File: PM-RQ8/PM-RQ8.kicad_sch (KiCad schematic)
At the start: 33 parts, among them J1 2EDGK-5.08-02P, J10 2EDGR-5.08-18P, J11 Shunt 2.54 Open Top, J12 PinHeader_P2.54_01x03_SMD_Str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, J13 PinHeader_P2.54_01x03_SMD_Str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, J14 PinHeader_P2.54_01x03_SMD_Str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, J15 FemaleHeader P2.54 02x08 THT 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, J16 Shunt 2.54 Open Top, J17 Shunt 2.54 Open Top, J18 2EDGK-5.08-02P, J2 2EDGK-5.08-02P, J3 2EDGK-5.08-02P, J4 2EDGK-5.08-02P, J5 2EDGK-5.08-02P, J6 2EDGK-5.08-02P, J7 2EDGK-5.08-02P, J8 2EDGK-5.08-02P, J9 Conn_01x04_Pin, K1 G5NB-1A-E-DC5, K2 G5NB-1A-E-DC5, K3 G5NB-1A-E-DC5, K4 G5NB-1A-E-DC5, K5 G5NB-1A-E-DC5, K6 G5NB-1A-E-DC5, K7 G5NB-1A-E-DC5, K8 G5NB-1A-E-DC5, U1 ULN2803A, U2 PCA9555PW, U4 64900001039

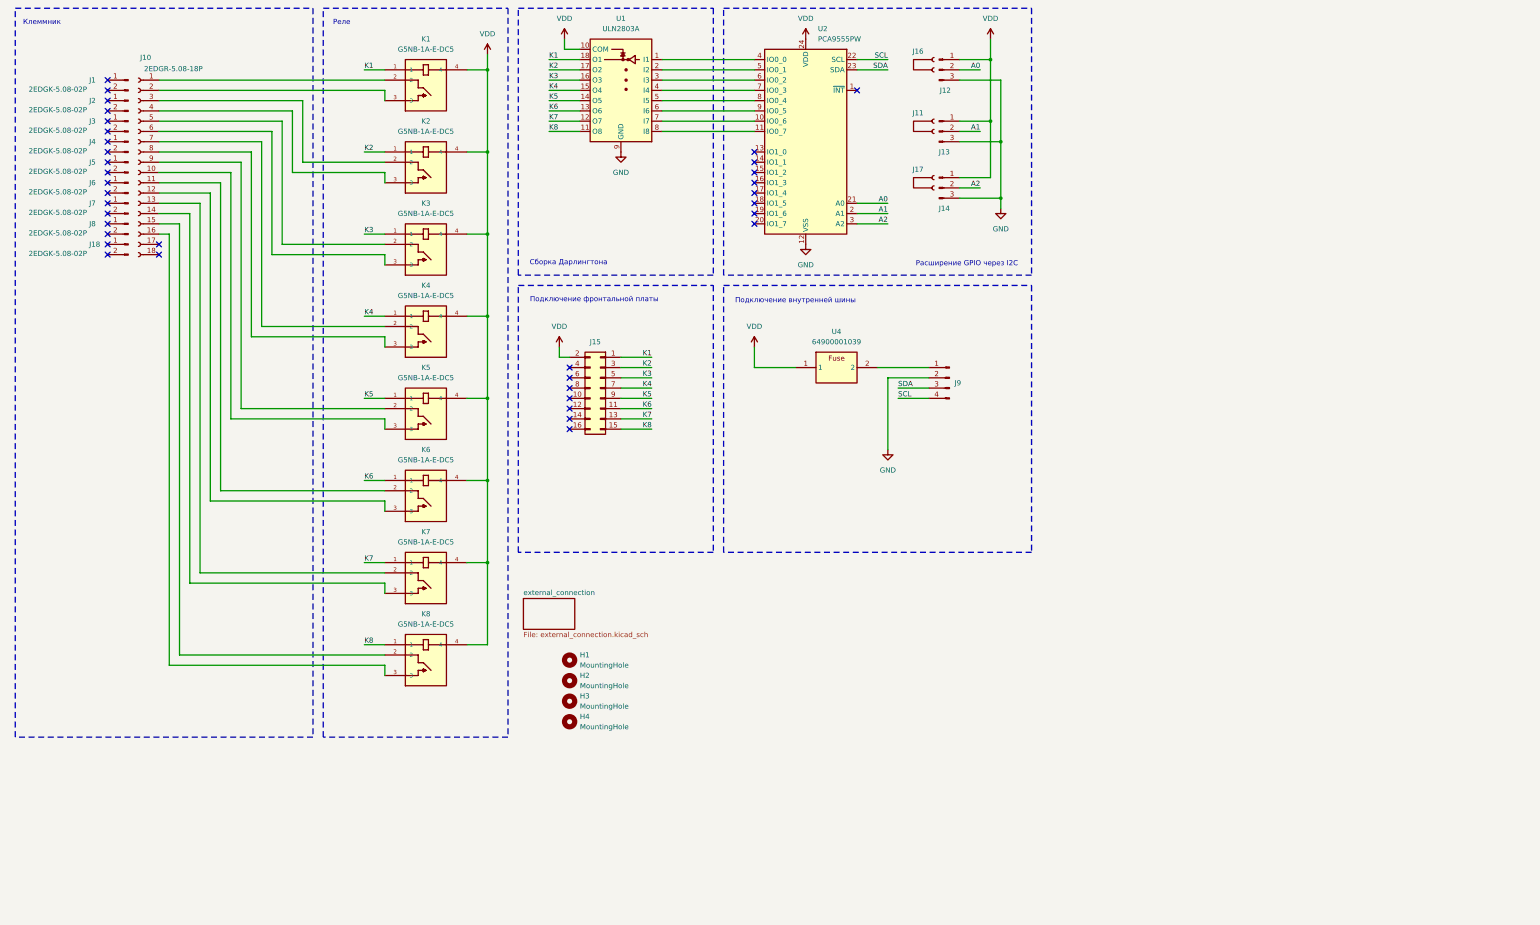
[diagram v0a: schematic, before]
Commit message: send to nextpcb
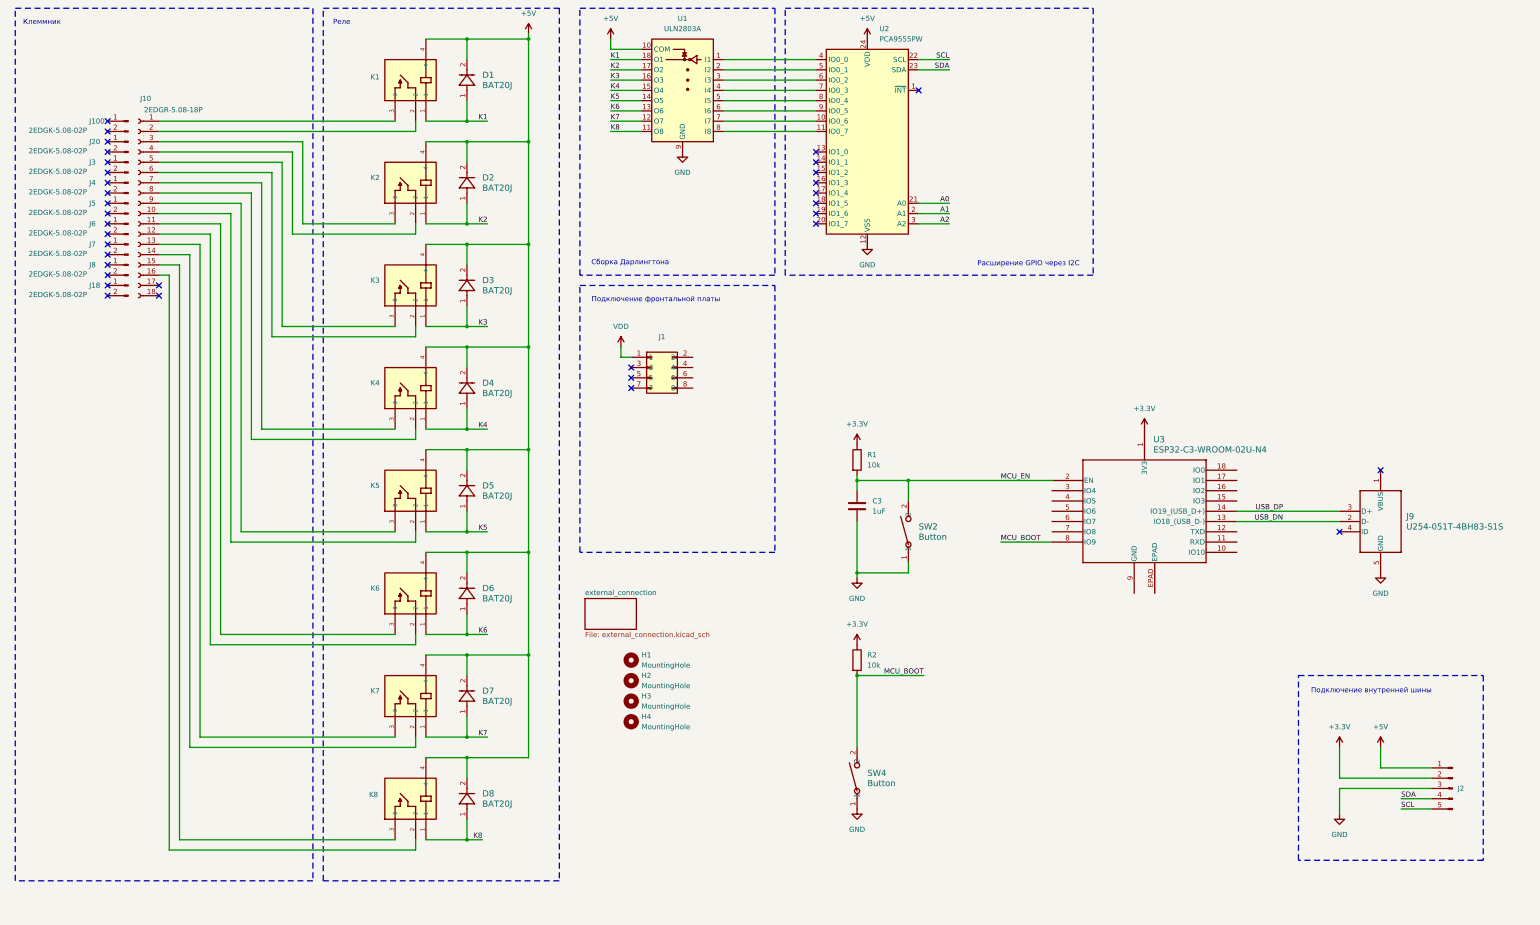
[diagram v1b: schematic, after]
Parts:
- removed J11, J16, J17: Shunt 2.54 Open Top, symbol kicad_inventree_lib:Shunt 2.54 Open Top
- removed J12, J13, J14: PinHeader_P2.54_01x03_SMD_Straight, Connector_PinHeader_2.54mm:PinHeader_1x03_P2.54mm_Vertical_SMD_Pin1Left, symbol kicad_inventree_lib:PinHeader P2.54 01x03 SMD Straight
- removed J15: FemaleHeader P2.54 02x08 THT Straight, Connector_PinSocket_2.54mm:PinSocket_2x08_P2.54mm_Vertical, symbol kicad_inventree_lib:FemaleHeader P2.54 02x08 THT Straight
- removed J9: Conn_01x04_Pin, Connector_PinHeader_2.54mm:PinHeader_1x04_P2.54mm_Horizontal, symbol kicad_inventree_lib:PinHeader P2.54 01x04 THT Angle
- removed U4: 64900001039, NextPCB:Fuseholder, symbol kicad_inventree_lib:Fuseholder
- added C3: 1uF, Capacitor_SMD:C_1206_3216Metric_Pad1.33x1.80mm_HandSolder, symbol kicad_inventree_lib:C_1uF_50V_1206
- added D1, D2, D3, D4, D5, D6, D7, D8: BAT20J, kicad_inventree_lib:SOD-323_STM-M, symbol kicad_inventree_lib:BAT20J
- added J1: ~, kicad_inventree_lib:PM-front-02x04, symbol kicad_inventree_lib:PM-front-02x04
- added J2: PinHeader_01x05_P2.54_THT_angle, Connector_PinHeader_2.54mm:PinHeader_1x05_P2.54mm_Horizontal, symbol kicad_inventree_lib:PinHeader_01x05_P2.54_THT_angle
- added J9: U254-051T-4BH83-S1S, kicad_inventree_lib:CONN5_H83-S1S_XKB, symbol kicad_inventree_lib:XKG_U254-051T-4BH83-S1S
- added R1, R2: 10k, Resistor_SMD:R_1206_3216Metric_Pad1.30x1.75mm_HandSolder, symbol kicad_inventree_lib:R_10k_1206_1%
- added SW2, SW4: Button, kicad_inventree_lib:SW_TS-1088_XNP-M, symbol kicad_inventree_lib:TS-1088-AR02016
- added U3: ESP32-C3-WROOM-02U-N4, ESP32-C3-WROOM-02U_EXP, symbol kicad_inventree_lib:ESP32-C3-WROOM-02U-N4
- renumbered J1 to J100, J2 to J20
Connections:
- net GND: now also C3.2, J2.3 (Pin_3), J9.5 (GND), SW2.1, SW4.1
- net K1: now also D1.1
- net K2: now also D2.1
- net K3: now also D3.1
- net K4: now also D4.1
- net K5: now also D5.1
- net K6: now also D6.1
- net K7: now also D7.1
- net K8: now also D8.1
- net SCL: now also J2.5 (Pin_5)
- net SDA: now also J2.4 (Pin_4)
- net VDD: now also J1.1; no longer K1.4, K2.4, K3.4, K4.4, K5.4, K6.4, K7.4, K8.4, U1.10 (COM), U2.24 (VDD)
- net at K5.2: now also J10.10 (Pin_10); no longer J10.9 (Pin_9)
- net at K5.3: now also J10.9 (Pin_9); no longer J10.10 (Pin_10)
- net at K3.2: now also J10.6 (Pin_6); no longer J10.5 (Pin_5)
- net at K3.3: now also J10.5 (Pin_5); no longer J10.6 (Pin_6)
- net at K8.2: now also J10.16 (Pin_16); no longer J10.15 (Pin_15)
- net at K8.3: now also J10.15 (Pin_15); no longer J10.16 (Pin_16)
- net at K2.2: now also J10.4 (Pin_4); no longer J10.3 (Pin_3)
- net at K2.3: now also J10.3 (Pin_3); no longer J10.4 (Pin_4)
- net at K4.2: now also J10.8 (Pin_8); no longer J10.7 (Pin_7)
- net at K4.3: now also J10.7 (Pin_7); no longer J10.8 (Pin_8)
- net at K1.2: now also J10.2 (Pin_2); no longer J10.1 (Pin_1)
- net at K1.3: now also J10.1 (Pin_1); no longer J10.2 (Pin_2)
- net at J10.11 (Pin_11): now also K6.3; no longer K6.2
- net at J10.12 (Pin_12): now also K6.2; no longer K6.3
- net at J10.13 (Pin_13): now also K7.3; no longer K7.2
- net at J10.14 (Pin_14): now also K7.2; no longer K7.3
- new net +3.3V: J2.2 (Pin_2), R1.1, R2.1, U3.1 (3V3)
- new net +5V: D1.2, D2.2, D3.2, D4.2, D5.2, D6.2, D7.2, D8.2, J2.1 (Pin_1), K1.4, K2.4, K3.4, K4.4, K5.4, K6.4, K7.4, K8.4, U1.10 (COM), U2.24 (VDD)
- new net MCU_BOOT: R2.2, SW4.2, U3.8 (IO9)
- new net MCU_EN: C3.1, R1.2, SW2.2, U3.2 (EN)
- new net USB_DN: J9.2 (D-), U3.13 (IO18_(USB_D-))
- new net USB_DP: J9.3 (D+), U3.14 (IO19_(USB_D+))
- no-connect marks 36 -> 34
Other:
- moved on the sheet: H1, H2, H3, H4, J10, J100, J18, J20, J3, J4, J5, J6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

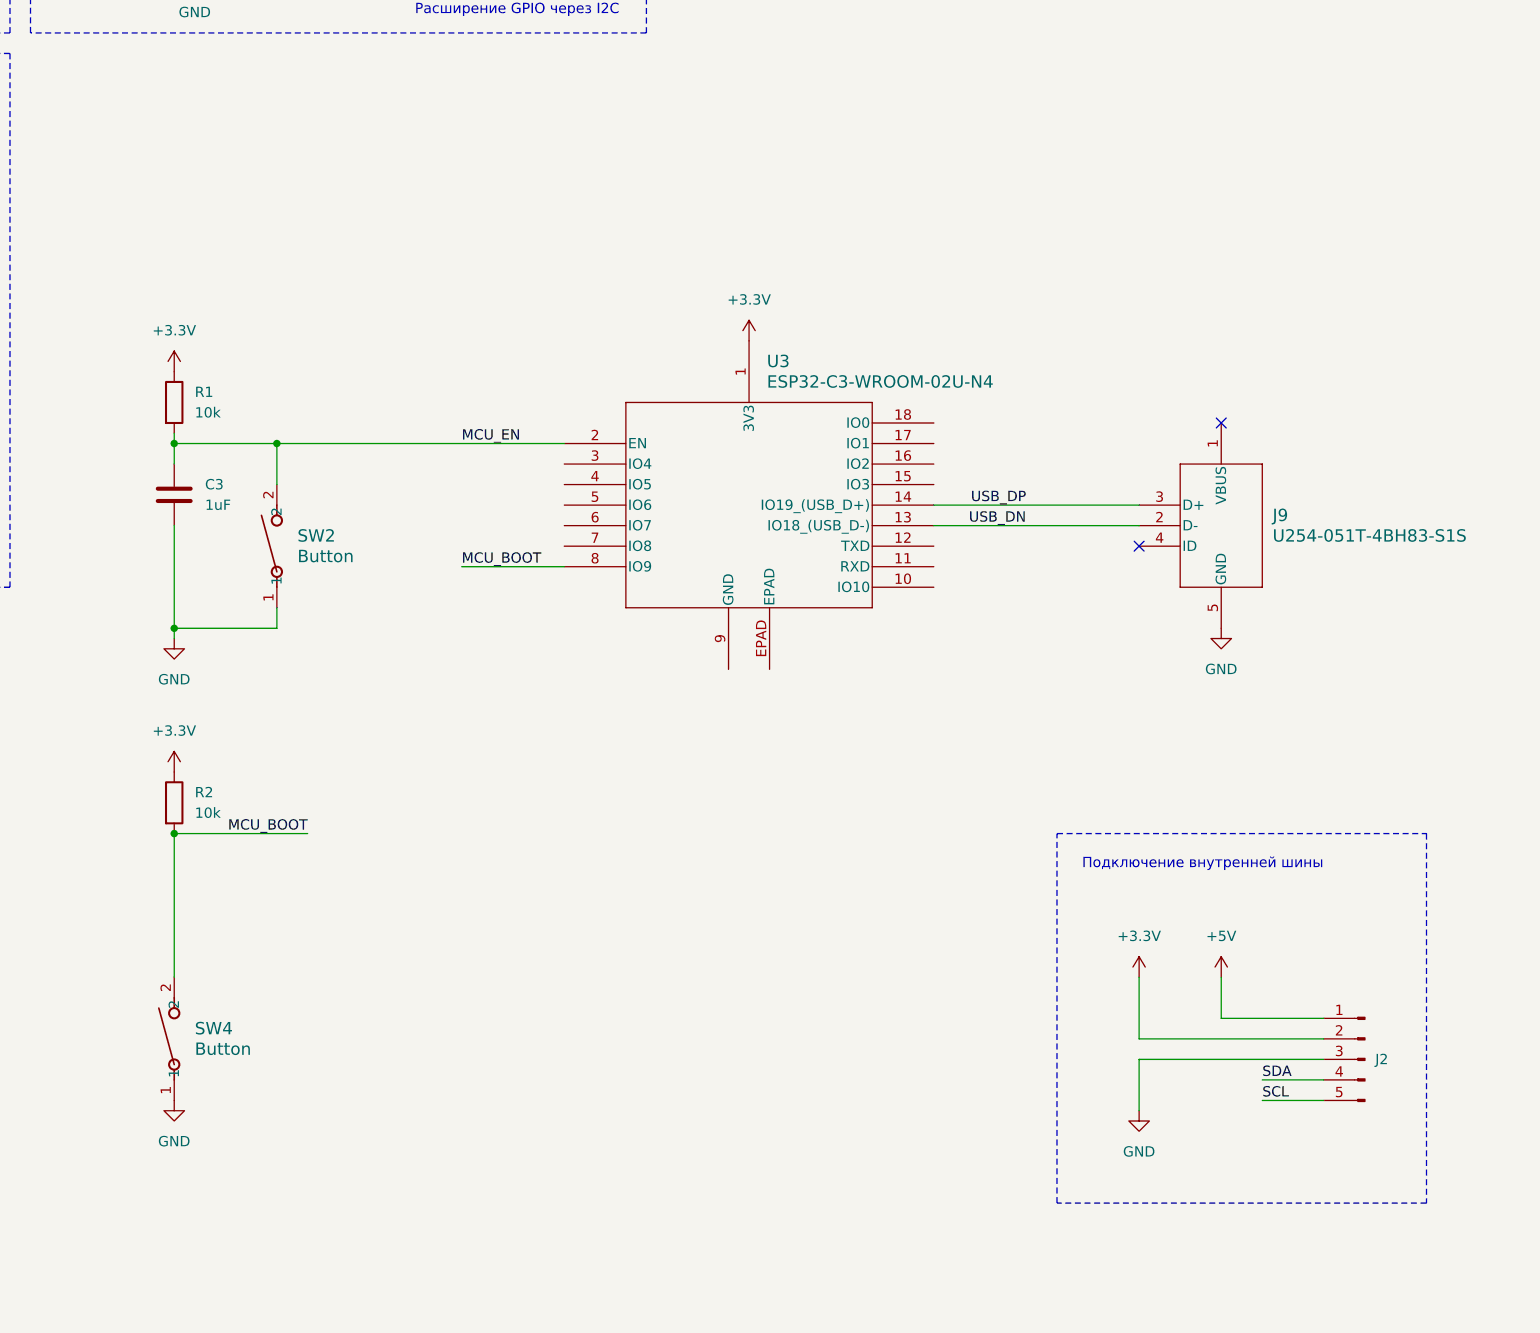
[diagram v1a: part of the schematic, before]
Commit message: PM-PS
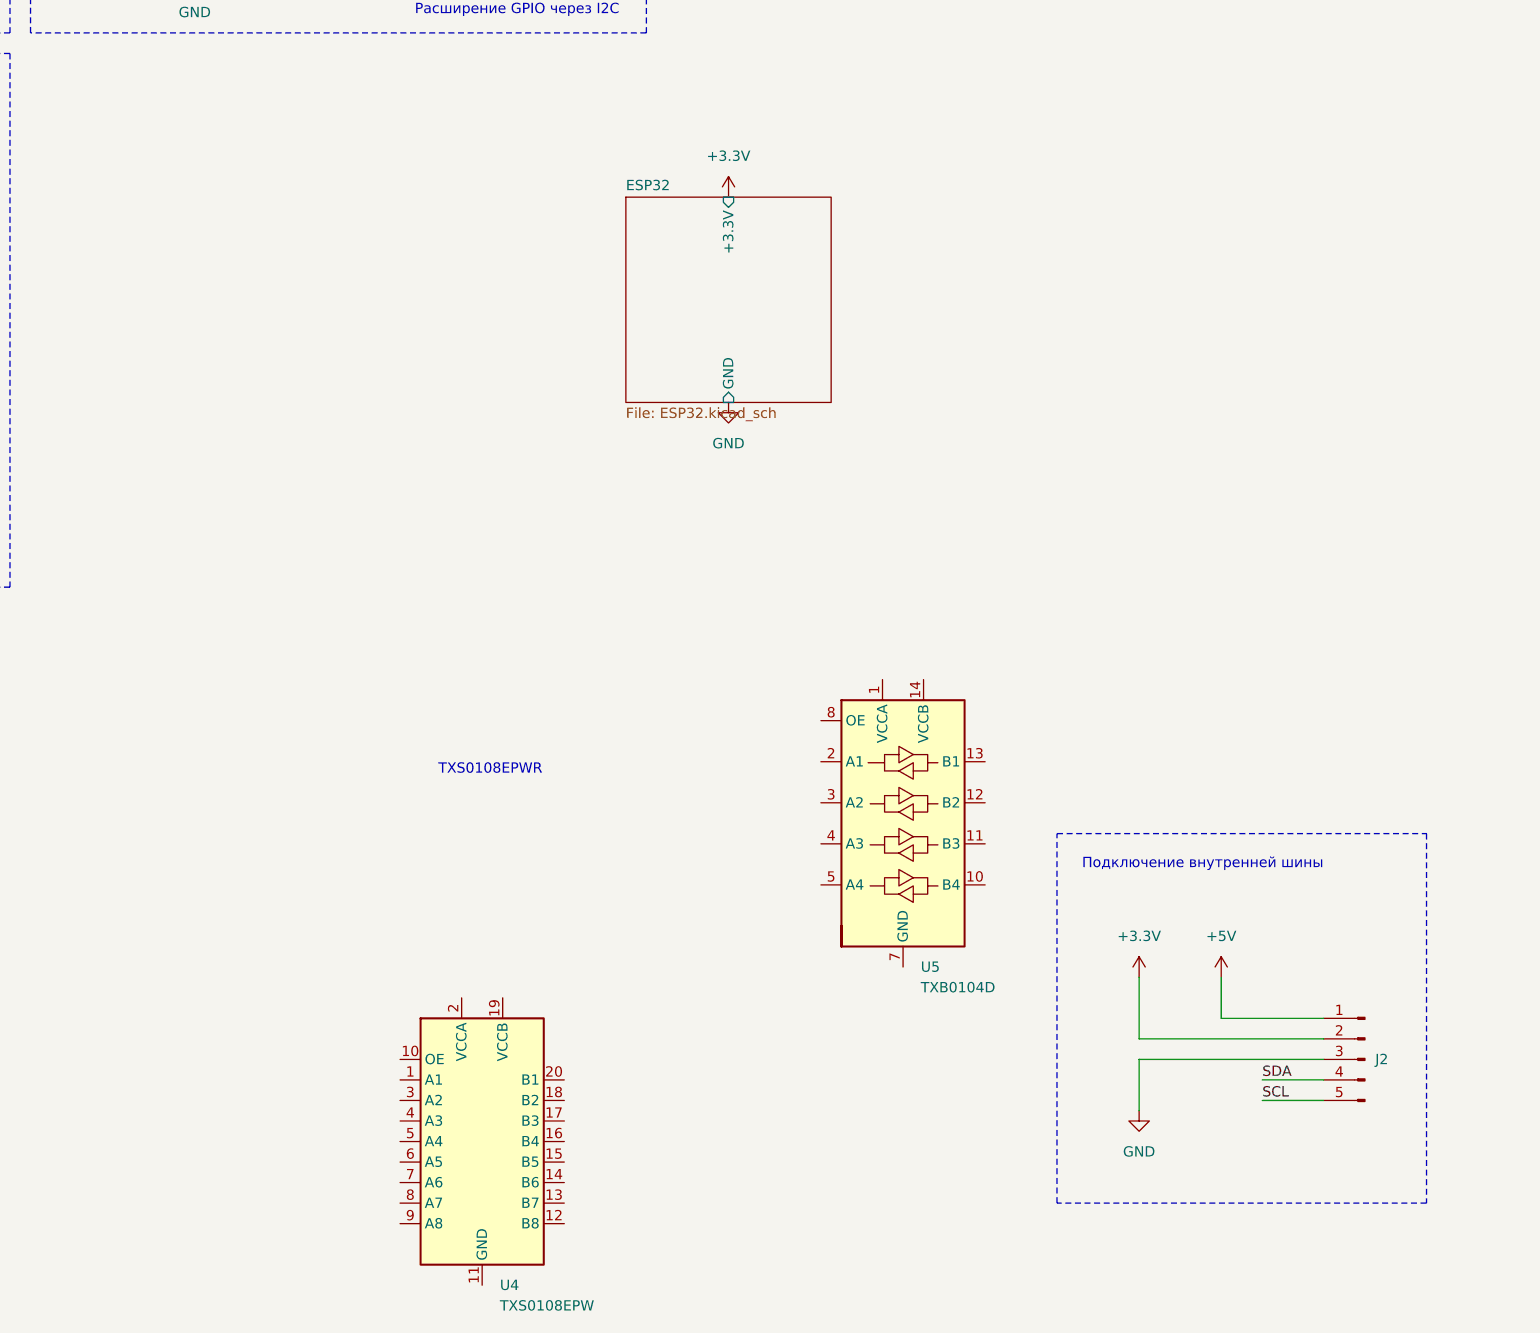
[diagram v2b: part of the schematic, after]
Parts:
- removed C3: 1uF, Capacitor_SMD:C_1206_3216Metric_Pad1.33x1.80mm_HandSolder, symbol kicad_inventree_lib:C_1uF_50V_1206
- removed J9: U254-051T-4BH83-S1S, kicad_inventree_lib:CONN5_H83-S1S_XKB, symbol kicad_inventree_lib:XKG_U254-051T-4BH83-S1S
- removed R1, R2: 10k, Resistor_SMD:R_1206_3216Metric_Pad1.30x1.75mm_HandSolder, symbol kicad_inventree_lib:R_10k_1206_1%
- removed SW2, SW4: Button, kicad_inventree_lib:SW_TS-1088_XNP-M, symbol kicad_inventree_lib:TS-1088-AR02016
- removed U3: ESP32-C3-WROOM-02U-N4, ESP32-C3-WROOM-02U_EXP, symbol kicad_inventree_lib:ESP32-C3-WROOM-02U-N4
- added U4: TXS0108EPW, Package_SO:TSSOP-20_4.4x6.5mm_P0.65mm, symbol Logic_LevelTranslator:TXS0108EPW
- added U5: TXB0104D, Package_SO:SOIC-14_3.9x8.7mm_P1.27mm, symbol Logic_LevelTranslator:TXB0104D
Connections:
- no-connect marks 34 -> 32
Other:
- added sheet ESP32 (ESP32.kicad_sch)
- note added: "TXS0108EPWR"
